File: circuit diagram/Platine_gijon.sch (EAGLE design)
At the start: 9 parts, among them M1 MOTOR, U1 MD22

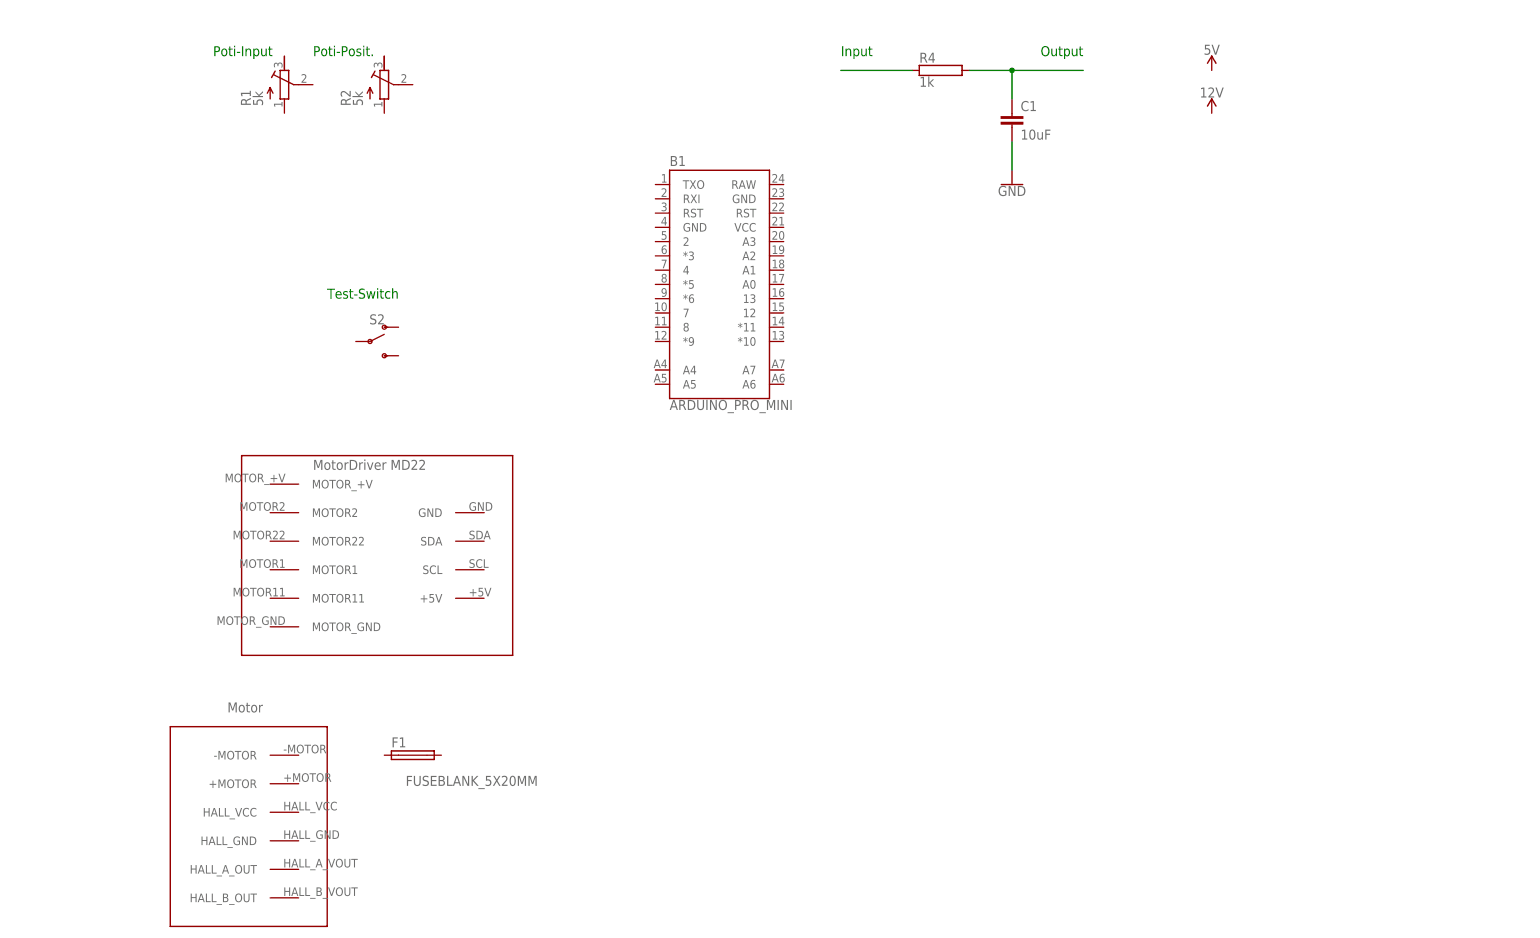
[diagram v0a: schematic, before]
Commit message: Casi Termino :)
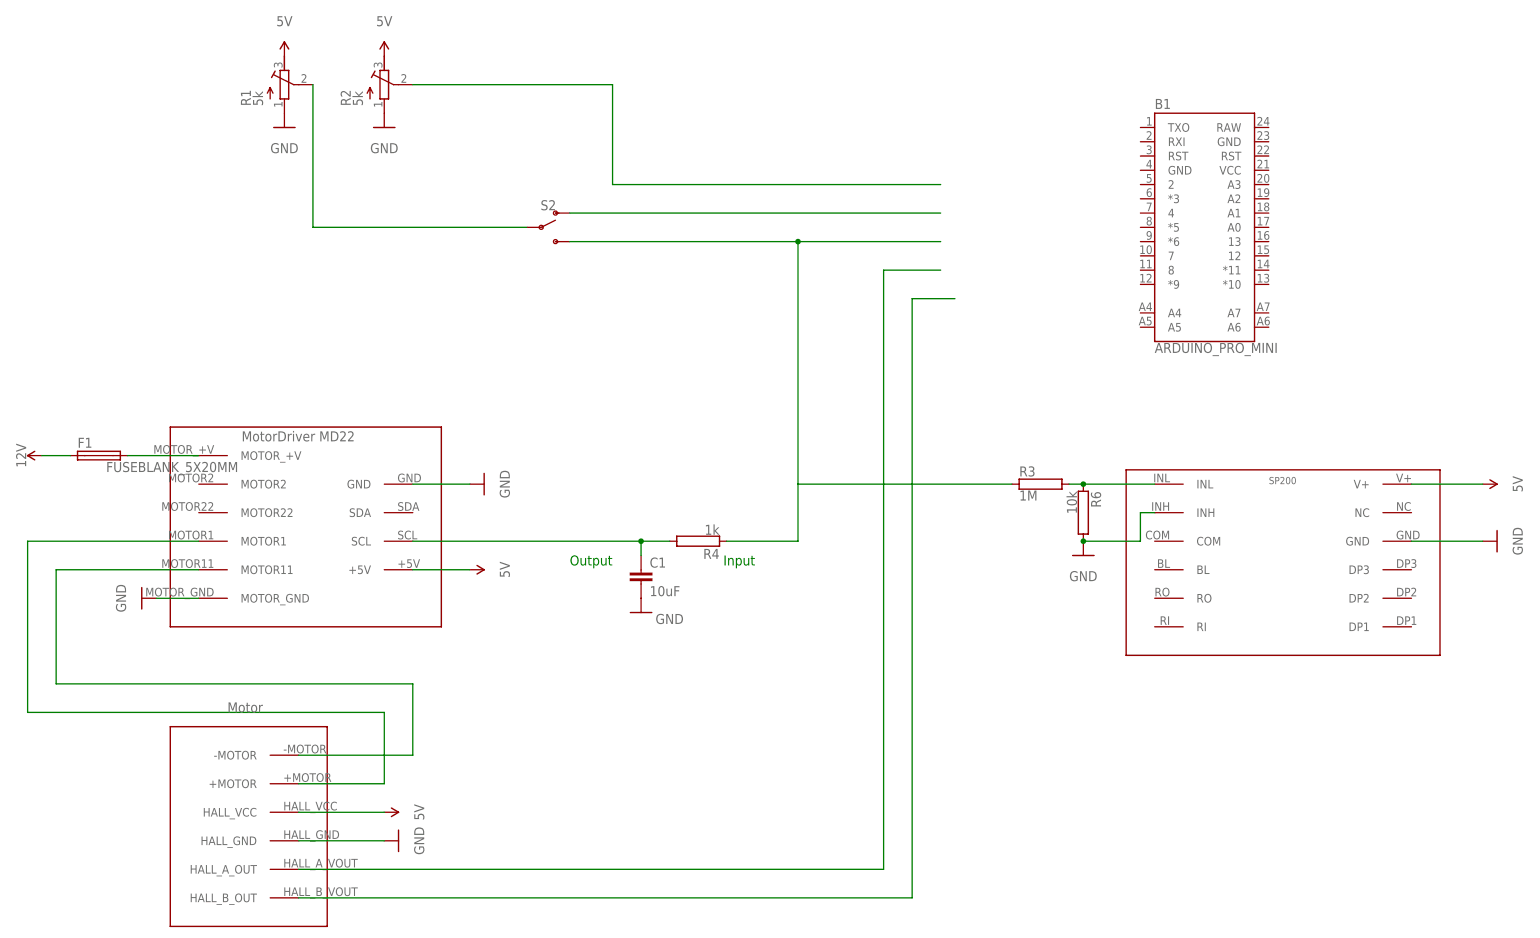
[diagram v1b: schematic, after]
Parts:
- added R3: 1M, resistor-power:RAC01
- added R6: 10k, resistor-power:RAC01
- added U$1: SP200, lib_gijon:SP200
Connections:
- new net 12V: F1.1
- new net 5V: M1.HALL_VCC, R1.E, R2.E, U$1.V+, U1.+5V
- new net N$1: F1.2, U1.MOTOR_+V
- new net N$10: M1.HALL_A_OUT
- new net N$11: M1.HALL_B_OUT
- new net N$2: M1.-MOTOR, U1.MOTOR11
- new net N$5: M1.+MOTOR, U1.MOTOR1
- new net N$6: R1.S, S2.P
- new net N$7: R3.2, R6.1, U$1.INL
- new net N$8: S2.O
- new net N$9: R2.S
- net GND: now also M1.HALL_GND, R1.A, R2.A, R6.2, U$1.GND, U$1.INH, U1.GND, U1.MOTOR_GND
- net N$3: now also U1.SCL
- net N$4: now also R3.1, S2.S
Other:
- note added: "2, ChannelB"
- note added: "3, ChannelA"
- note added: "6, PWM_Output"
- note added: "A0, Input Speed"
- note added: "A3, Poti. - Postion"
- moved on the sheet: B1, C1, F1, R4, S2
